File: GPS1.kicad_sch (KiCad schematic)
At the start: 12 parts, among them J7 GPS_ANT_0, U4 MAX-M10S-00B

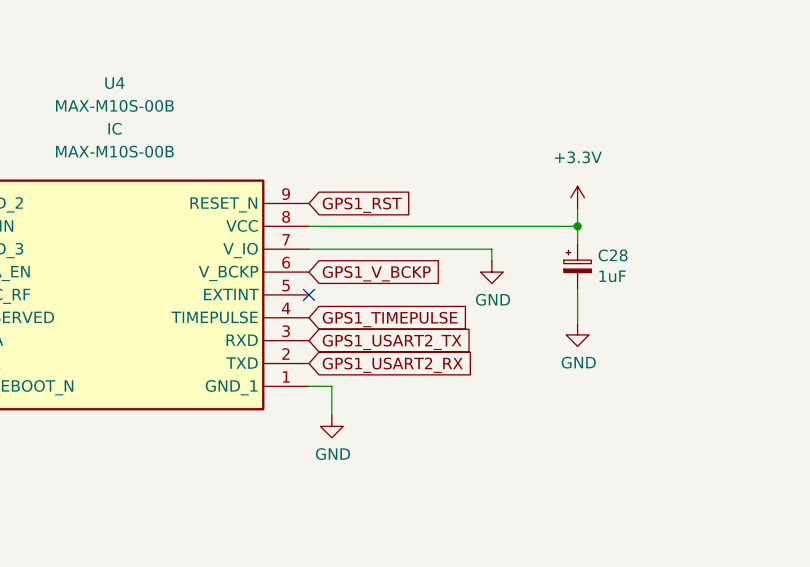
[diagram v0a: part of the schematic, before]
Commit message: Finished M10
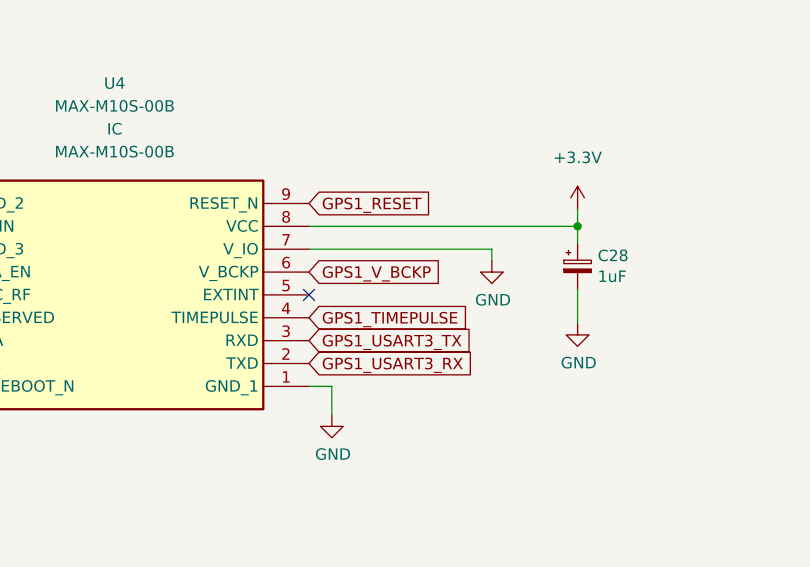
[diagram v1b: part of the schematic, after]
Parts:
- C25: footprint Capacitor_SMD:C_0805_2012Metric -> Capacitor_SMD:C_0402_1005Metric
- L3: footprint Inductor_SMD:L_0805_2012Metric -> Inductor_SMD:L_0402_1005Metric
- R15: footprint Resistor_SMD:R_0805_2012Metric -> Resistor_SMD:R_0402_1005Metric
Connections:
- net GPS1_RST renamed GPS1_RESET
- net GPS1_USART2_RX renamed GPS1_USART3_RX
- net GPS1_USART2_TX renamed GPS1_USART3_TX
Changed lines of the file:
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@@
     (stroke (width 0) (type default) (color 0 0 0 0))
   )
-  (global_label "GPS1_RST" (shape input) (at 115.57 57.785 0) (fields_autoplaced)
-    (effects (font (size 1.27 1.27)) (justify left))
-    (property "Intersheet References" "${INTERSHEET_REFS}" (id 0) (at 127.3569 57.7056 0)
-      (effects (font (size 1.27 1.27)) (justify left) hide)
-    )
-  )
-  (global_label "GPS1_USART2_RX" (shape input) (at 115.57 75.565 0) (fields_autoplaced)
+  (global_label "GPS1_USART3_RX" (shape input) (at 115.57 75.565 0) (fields_autoplaced)
     (effects (font (size 1.27 1.27)) (justify left))
     (property "Intersheet References" "${INTERSHEET_REFS}" (id 0) (at 134.4326 75.4856 0)
@@
     )
   )
-  (global_label "GPS1_USART2_TX" (shape input) (at 115.57 73.025 0) (fields_autoplaced)
+  (global_label "GPS1_USART3_TX" (shape input) (at 115.57 73.025 0) (fields_autoplaced)
     (effects (font (size 1.27 1.27)) (justify left))
     (property "Intersheet References" "${INTERSHEET_REFS}" (id 0) (at 134.1302 72.9456 0)
@@
     )
   )
+  (global_label "GPS1_RESET" (shape input) (at 115.57 57.785 0) (fields_autoplaced)
+    (effects (font (size 1.27 1.27)) (justify left))
+    (property "Intersheet References" "${INTERSHEET_REFS}" (id 0) (at 129.655 57.7056 0)
+      (effects (font (size 1.27 1.27)) (justify left) hide)
+    )
+  )
   (symbol (lib_id "power:GND") (at 69.215 140.97 0) (unit 1)
     (in_bom yes) (on_board yes)
@@
     (property "Reference" "R15" (id 0) (at 48.26 60.96 0))
     (property "Value" "10R" (id 1) (at 48.26 63.5 0))
-    (property "Footprint" "Resistor_SMD:R_0805_2012Metric" (id 2) (at 51.435 62.23 0)
+    (property "Footprint" "Resistor_SMD:R_0402_1005Metric" (id 2) (at 51.435 62.23 0)
       (effects (font (size 1.27 1.27)) hide)
     )
@@
       (effects (font (size 1.27 1.27)) (justify left))
     )
-    (property "Footprint" "Capacitor_SMD:C_0805_2012Metric" (id 2) (at 36.83 62.23 0)
+    (property "Footprint" "Capacitor_SMD:C_0402_1005Metric" (id 2) (at 36.83 62.23 0)
       (effects (font (size 1.27 1.27)) hide)
     )
@@
     (property "Reference" "L3" (id 0) (at 47.625 52.705 0))
     (property "Value" "27nH" (id 1) (at 47.625 54.61 0))
-    (property "Footprint" "Inductor_SMD:L_0805_2012Metric" (id 2) (at 51.435 52.705 0)
-      (effects (font (size 1.27 1.27)) hide)
-    )
+    (property "Footprint" "Inductor_SMD:L_0402_1005Metric" (id 2) (at 51.435 52.705 0)
+      (effects (font (size 1.27 1.27)) hide)
+    )
